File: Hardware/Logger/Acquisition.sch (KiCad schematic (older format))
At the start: 9 parts, among them J1 Conn_Coaxial, J2 Conn_Coaxial, J3 Conn_Coaxial, J4 Conn_Coaxial, J7 DB9_Female_MountingHoles

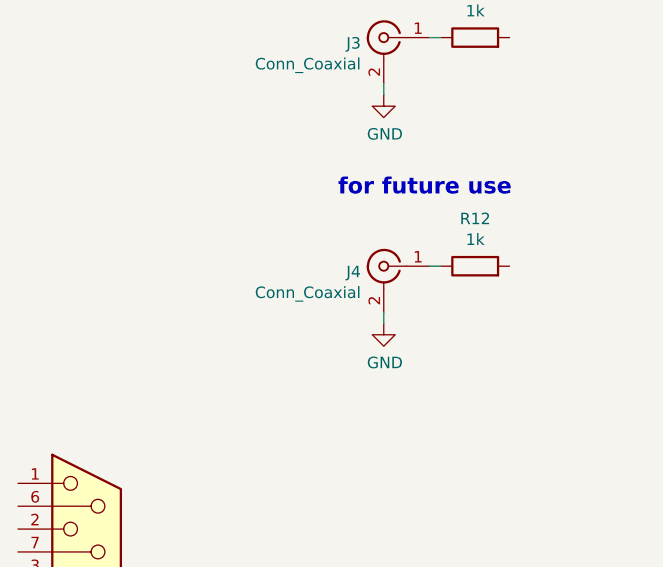
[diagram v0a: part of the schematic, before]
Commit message: fix #27, fix #30, fix #32
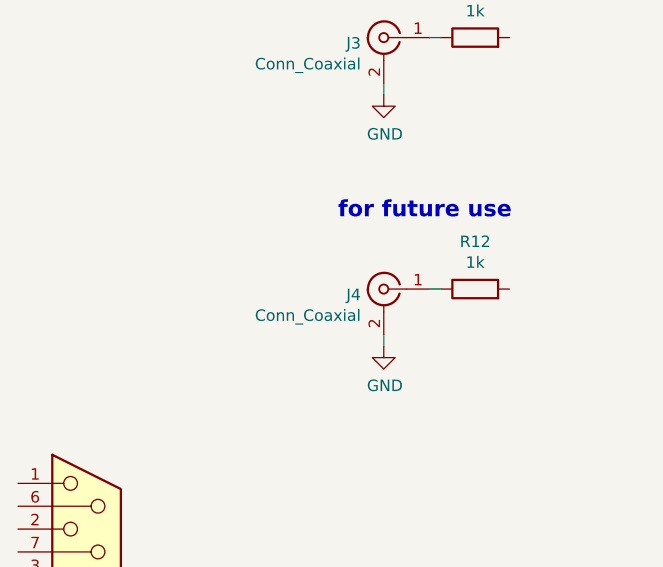
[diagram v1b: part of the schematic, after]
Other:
- moved on the sheet: J4, R12
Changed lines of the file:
@@
 $Descr A4 11693 8268
 encoding utf-8
-Sheet 3 6
+Sheet 3 7
 Title ""
 Date ""
@@
 Wire Wire Line
 	3700 4150 3750 4150
-Text Notes 3300 4850 0    71   ~ 14
+Text Notes 3300 4950 0    71   ~ 14
 for future use
 $Comp
 L Connector:Conn_Coaxial J?
 U 1 1 60F715EB
-P 3500 5150
+P 3500 5250
 AR Path="/60F715EB" Ref="J?"  Part="1"
 AR Path="/60F455B3/60F715EB" Ref="J4"  Part="1"
-F 0 "J4" H 3600 5125 50  0000 L CNN
-F 1 "Conn_Coaxial" H 3600 5034 50  0000 L CNN
-F 2 "Connector_Coaxial:SMA_Molex_73251-2200_Horizontal" H 3500 5150 50  0001 C CNN
-F 3 " ~" H 3500 5150 50  0001 C CNN
-	1    3500 5150
+F 0 "J4" H 3600 5225 50  0000 L CNN
+F 1 "Conn_Coaxial" H 3600 5134 50  0000 L CNN
+F 2 "Connector_Coaxial:SMA_Molex_73251-2200_Horizontal" H 3500 5250 50  0001 C CNN
+F 3 " ~" H 3500 5250 50  0001 C CNN
+	1    3500 5250
 	-1   0    0    -1
 $EndComp
@@
 L power:GND #PWR016
 U 1 1 60F715F1
-P 3500 5400
-F 0 "#PWR016" H 3500 5150 50  0001 C CNN
-F 1 "GND" H 3505 5227 50  0000 C CNN
-F 2 "" H 3500 5400 50  0001 C CNN
-F 3 "" H 3500 5400 50  0001 C CNN
-	1    3500 5400
+P 3500 5500
+F 0 "#PWR016" H 3500 5250 50  0001 C CNN
+F 1 "GND" H 3505 5327 50  0000 C CNN
+F 2 "" H 3500 5500 50  0001 C CNN
+F 3 "" H 3500 5500 50  0001 C CNN
+	1    3500 5500
 	1    0    0    -1
 $EndComp
 Wire Wire Line
-	3500 5350 3500 5400
+	3500 5450 3500 5500
 $Comp
 L Device:R R?
 U 1 1 60F715F8
-P 3900 5150
+P 3900 5250
 AR Path="/60F715F8" Ref="R?"  Part="1"
 AR Path="/60F39CF0/60F715F8" Ref="R?"  Part="1"
 AR Path="/60F455B3/60F715F8" Ref="R12"  Part="1"
-F 0 "R12" V 4107 5150 50  0000 C CNN
-F 1 "1k" V 4016 5150 50  0000 C CNN
-F 2 "Resistor_SMD:R_0805_2012Metric" V 3830 5150 50  0001 C CNN
-F 3 "~" H 3900 5150 50  0001 C CNN
-	1    3900 5150
+F 0 "R12" V 4107 5250 50  0000 C CNN
+F 1 "1k" V 4016 5250 50  0000 C CNN
+F 2 "Resistor_SMD:R_0805_2012Metric" V 3830 5250 50  0001 C CNN
+F 3 "~" H 3900 5250 50  0001 C CNN
+	1    3900 5250
 	0    -1   -1   0
 $EndComp
 Wire Wire Line
-	3700 5150 3750 5150
+	3700 5250 3750 5250
 $Comp
 L Connector:DB9_Female_MountingHoles J7
